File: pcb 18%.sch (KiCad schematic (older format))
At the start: 1 part

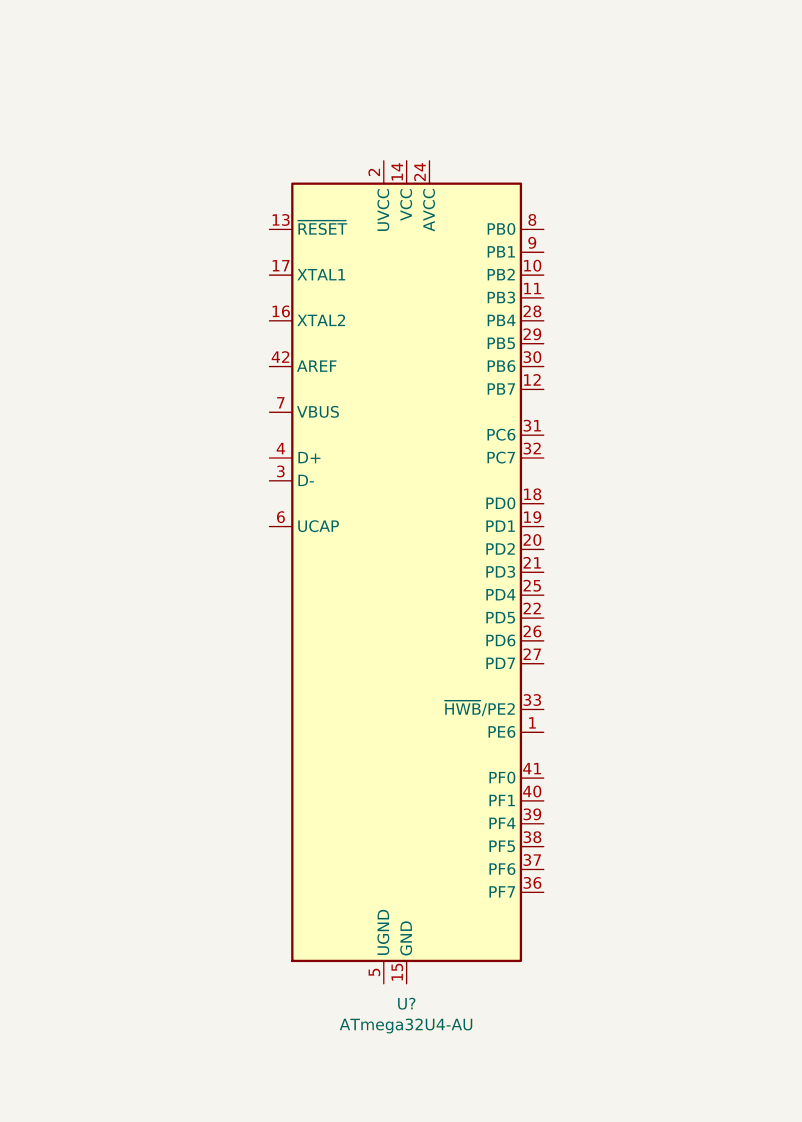
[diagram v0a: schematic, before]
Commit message: part 3 finish. Schematic things around the mcu
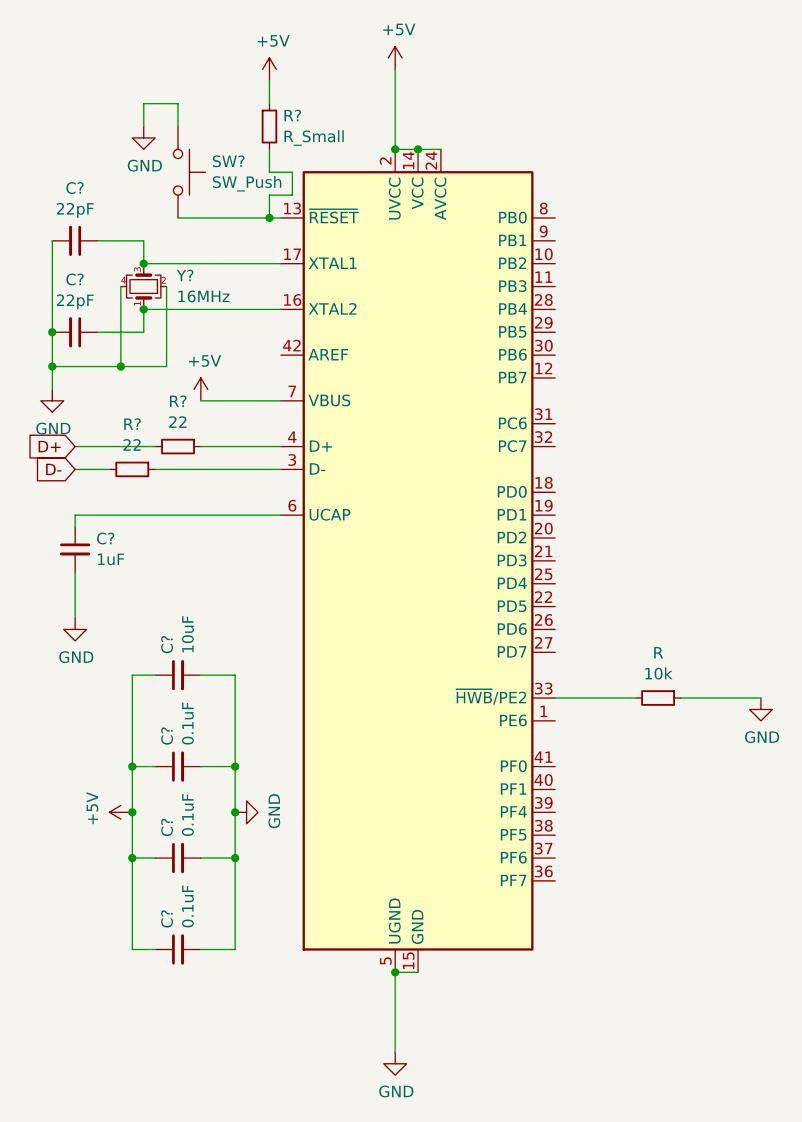
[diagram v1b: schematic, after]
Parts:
- added C?: 1uF, symbol Device:C_Small
- added C? (x3): 0.1uF, symbol Device:C_Small
- added C?: 10uF, symbol Device:C_Small
- added C? (x2): 22pF, symbol Device:C_Small
- added R: 10k, symbol Device:R_Small
- added R? (x2): 22, symbol Device:R_Small
- added R?: R_Small, symbol Device:R_Small
- added SW?: SW_Push, symbol Switch:SW_Push
- added Y?: 16MHz, symbol Device:Crystal_GND24_Small
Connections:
- net at U?.13 (~RESET): now also R?.2, SW?.2
- net +5V: now reaches U?.14 (VCC), U?.34 (VCC)
- net +5V: now also U?.2 (UVCC), U?.24 (AVCC), U?.44 (AVCC), U?.7 (VBUS), C?.1, C?.1, C?.1, C?.1, R?.1
- net GND: now reaches U?.15 (GND), U?.23 (GND), U?.35 (GND), U?.43 (GND)
- net GND: now also U?.5 (UGND), C?.2, C?.2, C?.2, C?.2, C?.2, C?.2, C?.2, R.1, SW?.1, Y?.2, Y?.4
- net at U?.16 (XTAL2): now also C?.1, Y?.1
- net at U?.17 (XTAL1): now also C?.1, Y?.3
- net at U?.3 (D-): now also R?.1
- net at U?.33 (~HWB~/PE2): now also R.2
- net at U?.4 (D+): now also R?.1
- net at U?.6 (UCAP): now also C?.1
- new net D+: R?.2
- new net D-: R?.2
